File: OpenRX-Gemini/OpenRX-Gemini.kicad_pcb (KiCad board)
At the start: 6 copper layers, 13.3 x 13.3 mm, 68 parts, among them T4 0900PC16J0042001E, T5 0900PC16J0042001E, U1 OW7EL89CENUYO3YLC-32M, U15 RFX2401C, U16 SKY13414-485LF, U17 RFX2401C, U18 SKY13414-485LF, U2 LR1121IMLTRT, U3 ESP32-C3FH4, U4 TS2306A 240GF MSM 9_C2976675, U6 TLV75533PDQNR, U9 LR1121IMLTRT, X1 CJ17-400001010B20

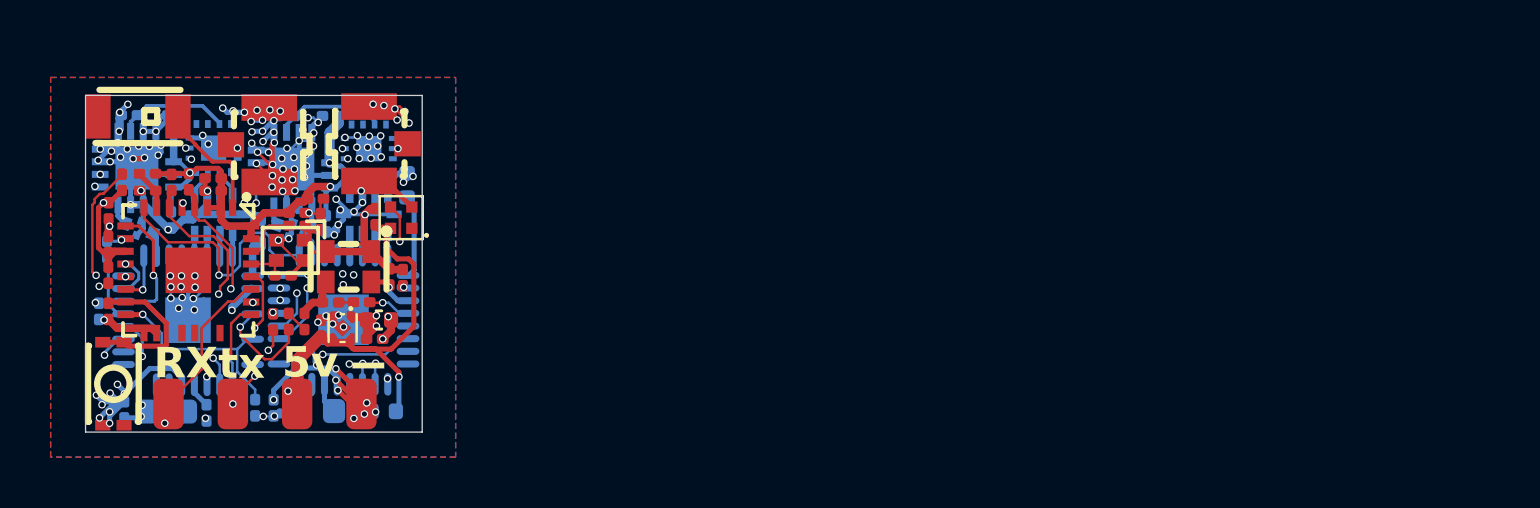
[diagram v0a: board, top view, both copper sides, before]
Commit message: pre-via-normalize snapshot
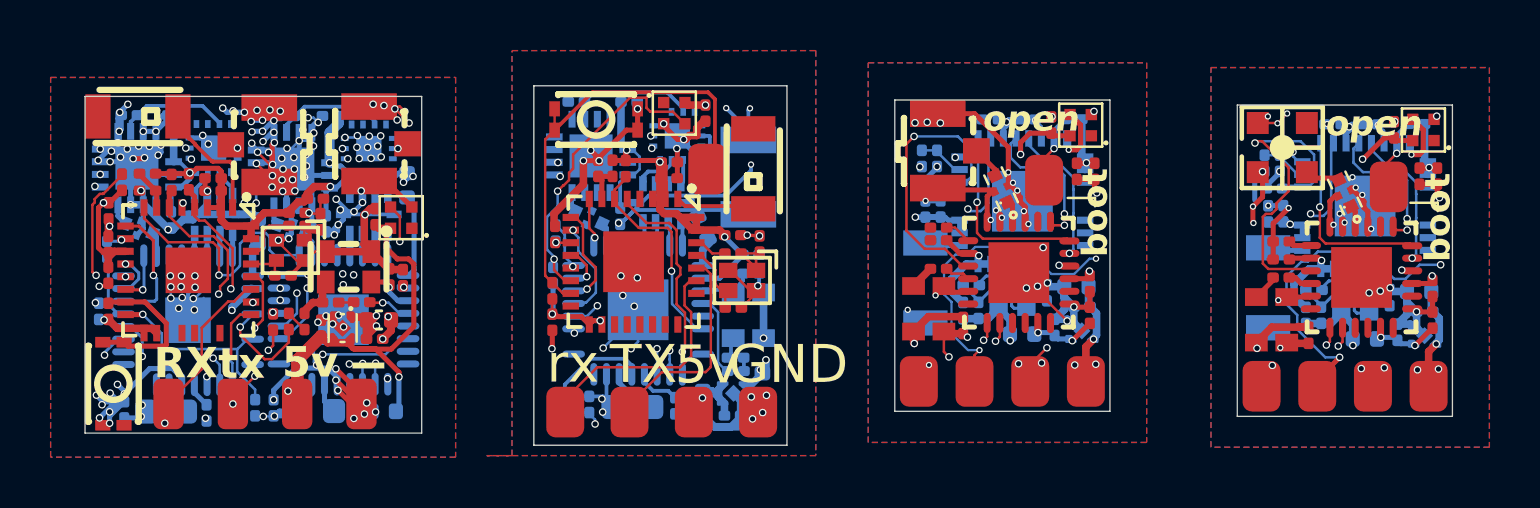
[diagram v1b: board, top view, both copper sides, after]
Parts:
- added AE1: 2450AT18A100E, OpenRX-Shared:ANT-SMD_L3.2-W1.6, F.Cu at (87.8, 47.6)
- added AE1: 2450AT18A100E, OpenRX-Shared:ANT-SMD_L3.2-W1.6, B.Cu at (108.1, 52.3)
- added AE1: 2450AT18A100E, OpenRX-Shared:ANT-SMD_L3.2-W1.6, B.Cu at (94.6, 52.1)
- added AE2: 47948-0001, OpenRX-Shared:ANT-SMD_47948-0001, F.Cu at (108.7, 46.8)
- added C1: 100nF, Capacitor_SMD:C_0201_0603Metric, F.Cu at (84.4, 47.4)
- added C1: 18pF, Capacitor_SMD:C_0201_0603Metric, B.Cu at (96.7, 53.2)
- added C1: 18pF, Capacitor_SMD:C_0201_0603Metric, B.Cu at (110.2, 53.4)
- added C10: 1uF, Capacitor_SMD:C_0201_0603Metric, B.Cu at (100.7, 53.1)
- added C10: 1uF, Capacitor_SMD:C_0201_0603Metric, B.Cu at (114.3, 53.3)
- added C11: 100nF, Capacitor_SMD:C_0201_0603Metric, F.Cu at (100.5, 47.7)
- added C11: 100nF, Capacitor_SMD:C_0201_0603Metric, F.Cu at (114.1, 47.9)
- added C11: 10uF, Capacitor_SMD:C_0402_1005Metric, B.Cu at (88.1, 56.2)
- added C12: 100nF, Capacitor_SMD:C_0201_0603Metric, B.Cu at (110.7, 45.9)
- added C12: 10uF, Capacitor_SMD:C_0402_1005Metric, B.Cu at (85.8, 56.9)
- added C12: 100nF, Capacitor_SMD:C_0201_0603Metric, B.Cu at (97.1, 45.7)
- added C13: 100nF, Capacitor_SMD:C_0201_0603Metric, F.Cu at (96.0, 53.8)
- added C13: 100nF, Capacitor_SMD:C_0201_0603Metric, F.Cu at (109.7, 54.2)
- added C13: 10pF, Capacitor_SMD:C_0201_0603Metric, B.Cu at (87.1, 55.6)
- added C14: 100nF, Capacitor_SMD:C_0201_0603Metric, F.Cu at (108.6, 51.2)
- added C14: 100nF, Capacitor_SMD:C_0201_0603Metric, F.Cu at (95.1, 50.4)
- added C14: 1uF, Capacitor_SMD:C_0201_0603Metric, B.Cu at (82.5, 49.5)
- added C15: 1uF, Capacitor_SMD:C_0201_0603Metric, B.Cu at (99.7, 53.9)
- added C15: 1uF, Capacitor_SMD:C_0201_0603Metric, B.Cu at (113.2, 54.1)
- added C15: 220pF, Capacitor_SMD:C_0201_0603Metric, B.Cu at (82.9, 45.0)
- added C16: 0.3pF, Capacitor_SMD:C_0201_0603Metric, B.Cu at (80.8, 45.0)
- added C16: 10uF, Capacitor_SMD:C_0402_1005Metric, B.Cu at (111.9, 54.3)
- added C16: 10uF, Capacitor_SMD:C_0402_1005Metric, B.Cu at (98.4, 54.1)
- added C17: 100nF, Capacitor_SMD:C_0201_0603Metric, F.Cu at (114.6, 52.3)
- added C17: 100nF, Capacitor_SMD:C_0201_0603Metric, F.Cu at (101.1, 52.1)
- added C18: 100nF, Capacitor_SMD:C_0201_0603Metric, F.Cu at (85.9, 45.4)
- added C18: 100nF, Capacitor_SMD:C_0201_0603Metric, F.Cu at (101.1, 53.4)
- added C18: 100nF, Capacitor_SMD:C_0201_0603Metric, F.Cu at (114.6, 53.6)
- added C19: 1uF, Capacitor_SMD:C_0201_0603Metric, F.Cu at (87.0, 50.2)
- added C19: 1nF, Capacitor_SMD:C_0201_0603Metric, F.Cu at (108.6, 51.9)
- added C19: 1nF, Capacitor_SMD:C_0201_0603Metric, F.Cu at (95.1, 51.6)
- added C2: 100nF, Capacitor_SMD:C_0201_0603Metric, F.Cu at (84.4, 48.0)
- added C2: 1uF, Capacitor_SMD:C_0201_0603Metric, B.Cu at (94.4, 47.2)
- added C2: 1uF, Capacitor_SMD:C_0201_0603Metric, B.Cu at (108.0, 47.4)
- added C20: 470nF, Capacitor_SMD:C_0201_0603Metric, F.Cu at (108.6, 50.5)
- added C20: 470nF, Capacitor_SMD:C_0201_0603Metric, F.Cu at (95.1, 49.9)
- added C20: 4.7uF, Capacitor_SMD:C_0402_1005Metric, B.Cu at (85.8, 49.9)
- added C21: 100nF, Capacitor_SMD:C_0201_0603Metric, B.Cu at (87.7, 51.0)
- added C22: 100nF, Capacitor_SMD:C_0201_0603Metric, B.Cu at (84.7, 57.0)
- added C23: 100nF, Capacitor_SMD:C_0201_0603Metric, B.Cu at (87.7, 51.8)
- added C24: 100nF, Capacitor_SMD:C_0201_0603Metric, B.Cu at (81.3, 56.9)
- added C3: 100nF, Capacitor_SMD:C_0201_0603Metric, F.Cu at (79.8, 53.7)
- added C3: 18pF, Capacitor_SMD:C_0201_0603Metric, B.Cu at (99.4, 52.5)
- added C3: 18pF, Capacitor_SMD:C_0201_0603Metric, B.Cu at (112.9, 52.7)
- added C4: 1uF, Capacitor_SMD:C_0201_0603Metric, B.Cu at (109.6, 53.4)
- added C4: 1uF, Capacitor_SMD:C_0201_0603Metric, B.Cu at (96.0, 53.2)
- added C4: 100nF, Capacitor_SMD:C_0201_0603Metric, B.Cu at (80.7, 56.9)
- added C5: 100nF, Capacitor_SMD:C_0201_0603Metric, F.Cu at (79.9, 50.2)
- added C5: 100nF, Capacitor_SMD:C_0201_0603Metric, B.Cu at (95.2, 49.2)
- added C5: 100nF, Capacitor_SMD:C_0201_0603Metric, B.Cu at (108.7, 49.4)
- added C6: 18pF, Capacitor_SMD:C_0201_0603Metric, F.Cu at (88.0, 50.6)
- added C6: 100nF, Capacitor_SMD:C_0201_0603Metric, B.Cu at (108.1, 49.4)
- added C6: 100nF, Capacitor_SMD:C_0201_0603Metric, B.Cu at (94.6, 49.2)
- added C7: 100nF, Capacitor_SMD:C_0201_0603Metric, F.Cu at (113.1, 46.1)
- added C7: 18pF, Capacitor_SMD:C_0201_0603Metric, F.Cu at (87.0, 53.1)
- added C7: 100nF, Capacitor_SMD:C_0201_0603Metric, F.Cu at (99.5, 45.9)
- added C8: 1uF, Capacitor_SMD:C_0201_0603Metric, F.Cu at (81.6, 47.6)
- added C8: 10uF, Capacitor_SMD:C_0402_1005Metric, B.Cu at (100.5, 52.3)
- added C8: 10uF, Capacitor_SMD:C_0402_1005Metric, B.Cu at (114.1, 52.5)
- added C9: 100nF, Capacitor_SMD:C_0201_0603Metric, F.Cu at (101.2, 47.7)
- added C9: 100nF, Capacitor_SMD:C_0201_0603Metric, F.Cu at (114.8, 47.9)
- added C9: 1uF, Capacitor_SMD:C_0201_0603Metric, B.Cu at (86.9, 57.4)
- added D1: XL-1010RGBC-WS2812B, OpenRX-Shared:LED-SMD_4P-L1.0-W1.0-TL_XL-1010RGBC-WS2812B, F.Cu at (114.2, 46.1)
- added D1: XL-1010RGBC-WS2812B, OpenRX-Shared:LED-SMD_4P-L1.0-W1.0-TL_XL-1010RGBC-WS2812B, F.Cu at (100.7, 45.9)
- added D1: XL-1010RGBC-WS2812B, OpenRX-Shared:LED-SMD_4P-L1.0-W1.0-TL_XL-1010RGBC-WS2812B, F.Cu at (84.6, 45.4)
- added FL1: 2450FM07D0034T, OpenRX-Shared:FILTER-SMD_4P-L1.0-W0.5-L, F.Cu at (111.1, 48.6)
- added FL1: 2450FM07D0034T, OpenRX-Shared:FILTER-SMD_4P-L1.0-W0.5-L, F.Cu at (97.5, 48.4)
- added FL1: 2450FM07D0034T, OpenRX-Shared:FILTER-SMD_4P-L1.0-W0.5-L, B.Cu at (81.3, 49.5)
- added JP1: U.FL-R-SMT-1(80), OpenRX-Shared:RF-SMD_FRF05002-JSS103M, F.Cu at (95.8, 46.9)
- added JP1: U.FL-R-SMT-1(80), OpenRX-Shared:RF-SMD_FRF05002-JSS103M, B.Cu at (86.8, 47.9)
- added L1: 10uH, Inductor_SMD:L_0603_1608Metric, B.Cu at (83.0, 57.0)
- added L1: 24nH, Inductor_SMD:L_0201_0603Metric, B.Cu at (109.9, 52.4)
- added L1: 24nH, Inductor_SMD:L_0201_0603Metric, B.Cu at (96.4, 52.2)
- added L2: 24nH, Inductor_SMD:L_0201_0603Metric, F.Cu at (87.0, 51.0)
- added OSC1: OW7EL89CENUNFAYLC-52M, OpenRX-Shared:OSC-SMD_4P-L2.0-W1.6-BL_TXC_7Z, F.Cu at (94.7, 53.1)
- added OSC1: OW7EL89CENUNFAYLC-52M, OpenRX-Shared:OSC-SMD_4P-L2.0-W1.6-BL_TXC_7Z, F.Cu at (108.2, 53.6)
- added R1: 10k, Resistor_SMD:R_0201_0603Metric, F.Cu at (82.2, 47.6)
- added R1: 10k, Resistor_SMD:R_0201_0603Metric, B.Cu at (95.0, 47.2)
- added R1: 10k, Resistor_SMD:R_0201_0603Metric, B.Cu at (108.6, 47.4)
- added R2: 10k, Resistor_SMD:R_0201_0603Metric, B.Cu at (108.3, 48.4)
- added R2: 10k, Resistor_SMD:R_0201_0603Metric, B.Cu at (94.8, 48.2)
- added R2: 10k, Resistor_SMD:R_0201_0603Metric, B.Cu at (80.0, 50.1)
- added R3: 10k, Resistor_SMD:R_0201_0603Metric, F.Cu at (79.8, 52.4)
- added R3: 10k, Resistor_SMD:R_0201_0603Metric, B.Cu at (98.6, 45.7)
- added R3: 10k, Resistor_SMD:R_0201_0603Metric, B.Cu at (112.1, 45.9)
- added R4: 10k, Resistor_SMD:R_0201_0603Metric, F.Cu at (82.7, 47.6)
- added R4: 10k, Resistor_SMD:R_0201_0603Metric, B.Cu at (100.4, 45.6)
- added R4: 10k, Resistor_SMD:R_0201_0603Metric, B.Cu at (114.0, 45.8)
- added R5: 10k, Resistor_SMD:R_0201_0603Metric, B.Cu at (79.8, 51.8)
- added R6: 220R, Resistor_SMD:R_0201_0603Metric, B.Cu at (87.1, 55.1)
- added T1: 0900PC16J0042001E, OpenRX-Shared:FILTER-SMD_10P-L2.0-W1.6-BL, B.Cu at (84.2, 49.0)
- added TP1: RX, OpenRX-Shared:SolderPad_1.2x2.0mm, F.Cu at (107.8, 56.2)
- added TP1: RX, OpenRX-Shared:SolderPad_1.2x2.0mm, F.Cu at (80.3, 57.2)
- added TP1: RX, OpenRX-Shared:SolderPad_1.2x2.0mm, F.Cu at (94.3, 56.0)
- added TP2: TX, OpenRX-Shared:SolderPad_1.2x2.0mm, F.Cu at (82.9, 57.2)
- added TP2: TX, OpenRX-Shared:SolderPad_1.2x2.0mm, F.Cu at (96.5, 56.0)
- added TP2: TX, OpenRX-Shared:SolderPad_1.2x2.0mm, F.Cu at (110.0, 56.2)
- added TP3: 5V, OpenRX-Shared:SolderPad_1.2x2.0mm, F.Cu at (100.9, 56.0)
- added TP3: 5V, OpenRX-Shared:SolderPad_1.2x2.0mm, F.Cu at (85.4, 57.2)
- added TP3: 5V, OpenRX-Shared:SolderPad_1.2x2.0mm, F.Cu at (114.4, 56.2)
- added TP4: GND, OpenRX-Shared:SolderPad_1.2x2.0mm, F.Cu at (98.7, 56.0)
- added TP4: GND, OpenRX-Shared:SolderPad_1.2x2.0mm, F.Cu at (88.0, 57.2)
- added TP4: GND, OpenRX-Shared:SolderPad_1.2x2.0mm, F.Cu at (112.2, 56.2)
- added TP5: Boot, OpenRX-Shared:SolderPad_1.2x2.0mm, F.Cu at (85.9, 47.6)
- added TP5: GND, OpenRX-Shared:SolderPad_1.2x2.0mm, F.Cu at (99.2, 48.1)
- added TP5: GND, OpenRX-Shared:SolderPad_1.2x2.0mm, F.Cu at (112.9, 48.3)
- added U1: ESP32-C3FH4, OpenRX-Shared:QFN-32_L5.0-W5.0-P0.50-TL-EP3.7, F.Cu at (83.0, 51.3)
- added U1: ESP32-C3FH4, OpenRX-Shared:QFN-32_L5.0-W5.0-P0.50-TL-EP3.7, B.Cu at (111.9, 49.1)
- added U1: ESP32-C3FH4, OpenRX-Shared:QFN-32_L5.0-W5.0-P0.50-TL-EP3.7, B.Cu at (98.4, 48.9)
- added U2: TLV75533PDQNR, OpenRX-Shared:X2SON-4_L1.0-W1.0-P0.65-TL-EP, B.Cu at (114.3, 54.2)
- added U2: TLV75533PDQNR, OpenRX-Shared:X2SON-4_L1.0-W1.0-P0.65-TL-EP, B.Cu at (87.0, 56.5)
- added U2: TLV75533PDQNR, OpenRX-Shared:X2SON-4_L1.0-W1.0-P0.65-TL-EP, B.Cu at (100.7, 54.0)
- added U3: SX1281IMLTRT, OpenRX-Shared:QFN-24_L4.0-W4.0-P0.50-TL-EP2.6, F.Cu at (111.8, 51.9)
- added U3: SX1281IMLTRT, OpenRX-Shared:QFN-24_L4.0-W4.0-P0.50-TL-EP2.6, F.Cu at (98.2, 51.7)
- added U3: TS2306A 240GF MSM 9_C2976675, OpenRX-Shared:SW-SMD_4P-L3.0-W2.0-P0.85-LS3.5, F.Cu at (81.5, 45.7)
- added U4: LR1121IMLTRT, OpenRX-Shared:QFN-32_L5.0-W5.0-P0.50-BL-EP3.7, B.Cu at (83.2, 53.2)
- added U5: OW7EL89CENUYO3YLC-32M, OpenRX-Shared:OSC-SMD_4P-L2.0-W1.6-BL_TXC_7Z, B.Cu at (87.6, 53.4)
- added U7: RFX2401C, OpenRX-Shared:QFN-16_L3.0-W3.0-P0.50-BL-EP1.7, B.Cu at (81.3, 47.1)
- added U8: SKY13414-485LF, OpenRX-Shared:QFN-14_L2.0-W2.0-P0.45-BL-EP, B.Cu at (84.8, 46.3)
- added X1: CJ17-400001010B20, OpenRX-Shared:CRYSTAL-SMD_4P-L1.6-W1.2-BL, F.Cu at (87.3, 52.0)
- added X1: CJ17-400001010B20, OpenRX-Shared:CRYSTAL-SMD_4P-L1.6-W1.2-BL, B.Cu at (98.0, 52.7)
- added X1: CJ17-400001010B20, OpenRX-Shared:CRYSTAL-SMD_4P-L1.6-W1.2-BL, B.Cu at (111.5, 52.9)
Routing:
- net GND: track 155.9 -> 296.8 mm, vias 136 -> 220
- net +3V3: track 50.4 -> 121.9 mm, vias 14 -> 42
- net +5V: track 17.7 -> 66.8 mm, vias 2 -> 12
- net Net-(U1-U0RXD): track 0.00 -> 32.2 mm, vias 0 -> 4
- net Net-(U1-U0TXD): track 0.00 -> 27.9 mm, vias 0 -> 2
- net /ESP32-C3 + LR1121 Mono/BUTTON: track 0.00 -> 18.2 mm
- net /ESP32-C3 + SX1281 Core/RST: track 0.00 -> 13.2 mm, vias 0 -> 1
- net /ESP32-C3 + LR1121 Mono/LED: track 0.00 -> 12.0 mm, vias 0 -> 2
- net /ESP32-C3 + SX1281 Core (UFL)/RST: track 0.00 -> 11.8 mm, vias 0 -> 1
- net /ESP32-C3 + LR1121 Mono/DIO8-1: track 0.00 -> 10.2 mm, vias 0 -> 2
- net /ESP32-C3 + SX1281 Core/DIO1: track 0.00 -> 10.0 mm, vias 0 -> 2
- net /ESP32-C3 + SX1281 Core (UFL)/DIO1: track 0.00 -> 10.0 mm, vias 0 -> 2
- net /ESP32-C3 + SX1281 Core/BUSY: track 0.00 -> 9.55 mm, vias 0 -> 2
- net /ESP32-C3 + LR1121 Mono/DIO7-1: track 0.00 -> 9.16 mm, vias 0 -> 2
- net /ESP32-C3 + SX1281 Core (UFL)/BUSY: track 0.00 -> 8.60 mm, vias 0 -> 2
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- added copper zone on In3.Cu, net +3V3
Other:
- board size 13.3 x 13.3 mm -> 54 x 14.2 mm
- board text added: "GND"
- board text added: "TX"
- board text added: "boot"
- board text added: "open"
- board text added: "rx"
